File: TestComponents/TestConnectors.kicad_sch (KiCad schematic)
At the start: 9 parts, among them J2-1 Conn_01x04_Male, J2-2 Conn_01x04_Male

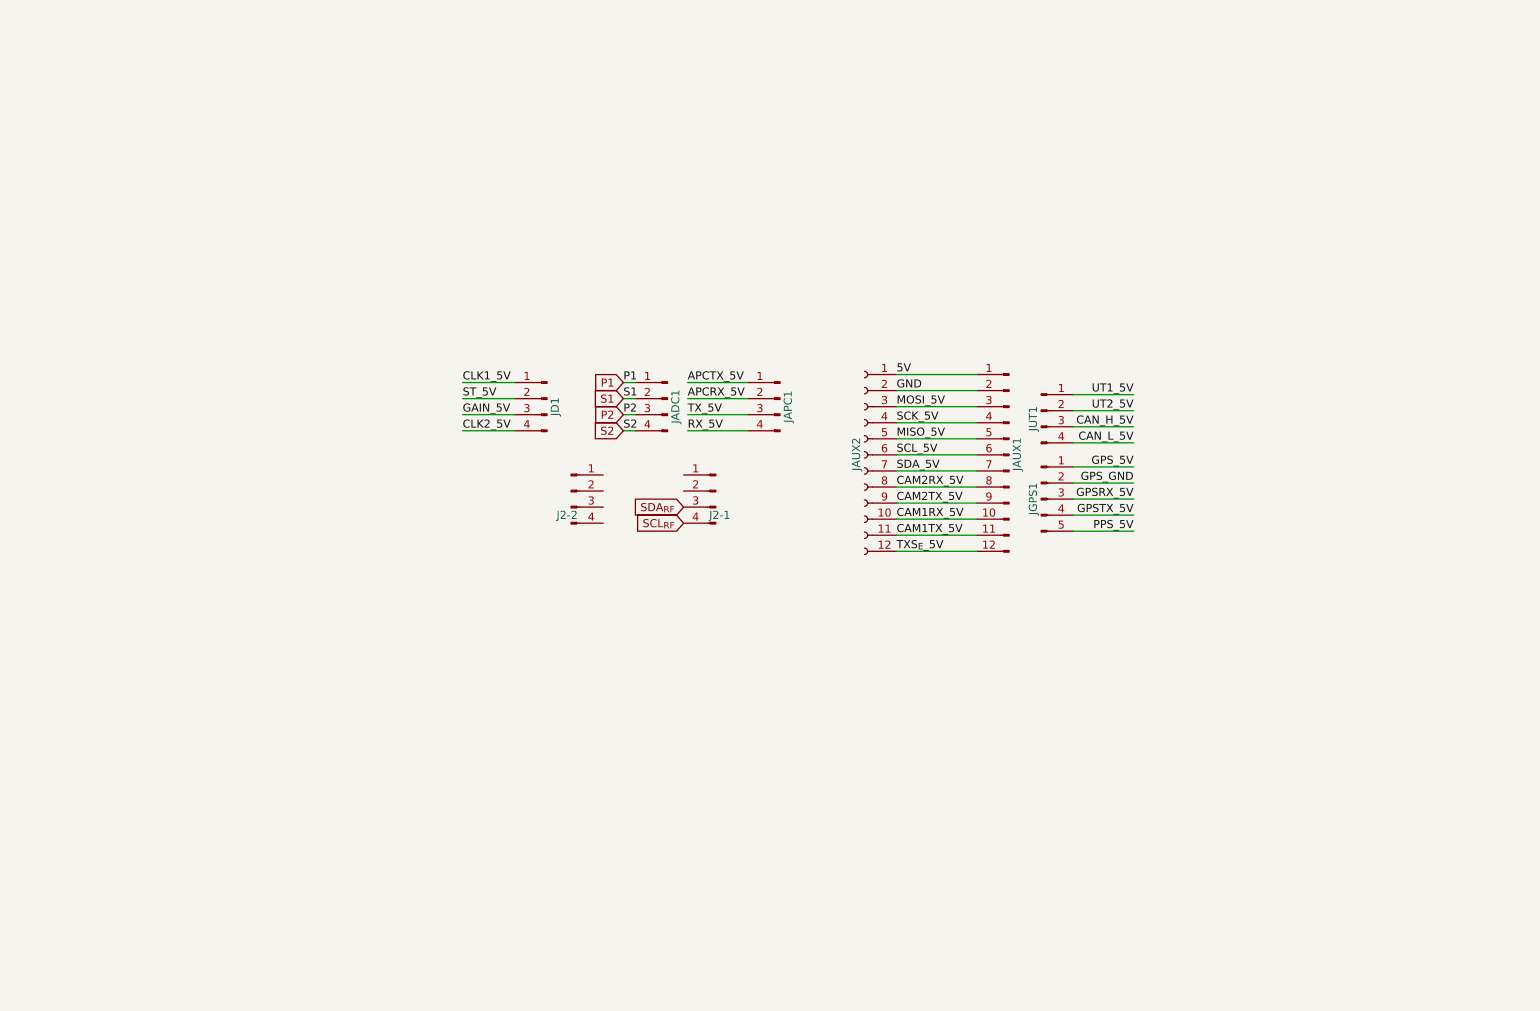
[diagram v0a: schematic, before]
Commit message: SpectDrone Development
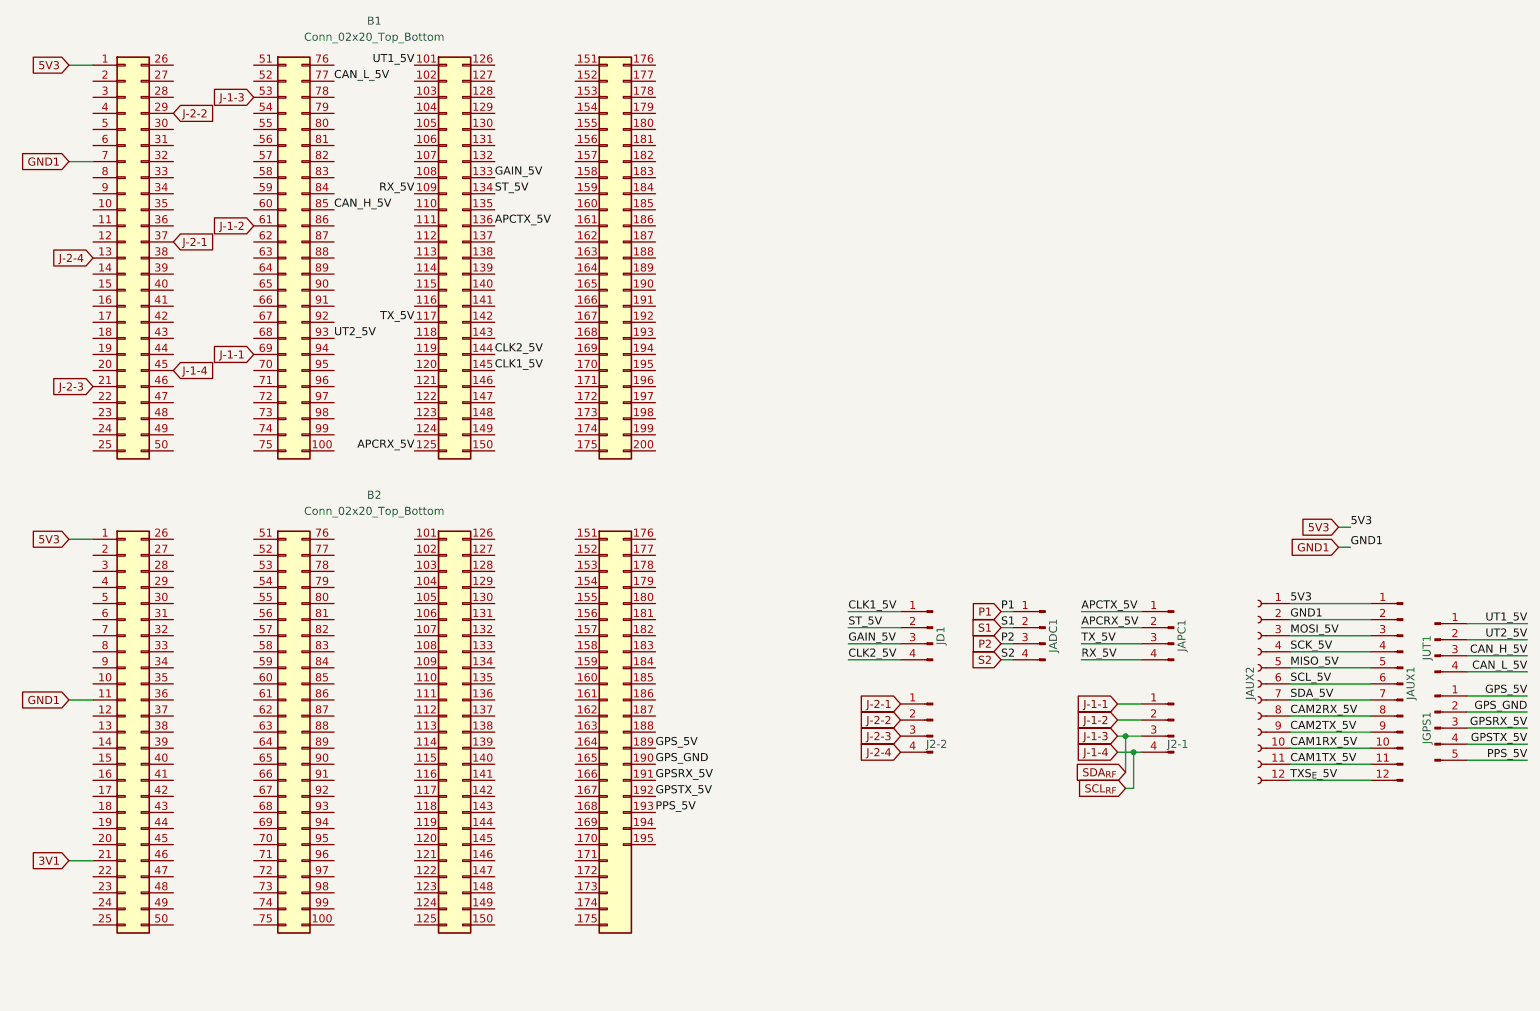
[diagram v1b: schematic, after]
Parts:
- added B1: Conn_02x20_Top_Bottom, Gardenuino Custom:PinHeader_CornerB1, symbol Connector_Generic:Conn_02x20_Top_Bottom
- added B2: Conn_02x20_Top_Bottom, Gardenuino Custom:PinHeader_CornerB2, symbol Connector_Generic:Conn_02x20_Top_Bottom
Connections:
- net APCRX_5V: now also B1.125 (Pin_125)
- net APCTX_5V: now also B1.136 (Pin_136)
- net CAN_H_5V: now also B1.85 (Pin_85)
- net CAN_L_5V: now also B1.77 (Pin_77)
- net CLK1_5V: now also B1.145 (Pin_145)
- net CLK2_5V: now also B1.144 (Pin_144)
- net GAIN_5V: now also B1.133 (Pin_133)
- net GPSRX_5V: now also B2.191 (Pin_191)
- net GPSTX_5V: now also B2.192 (Pin_192)
- net GPS_5V: now also B2.189 (Pin_189)
- net GPS_GND: now also B2.190 (Pin_190)
- net PPS_5V: now also B2.193 (Pin_193)
- net RX_5V: now also B1.109 (Pin_109)
- net ST_5V: now also B1.134 (Pin_134)
- net TX_5V: now also B1.117 (Pin_117)
- net UT1_5V: now also B1.101 (Pin_101)
- net UT2_5V: now also B1.93 (Pin_93)
- net J-2-1: now reaches J2-2.1 (Pin_1)
- net J-2-1: now also B1.37 (Pin_37)
- net J-2-2: now reaches J2-2.2 (Pin_2)
- net J-2-2: now also B1.29 (Pin_29)
- net J-2-3: now reaches J2-2.3 (Pin_3)
- net J-2-3: now also B1.21 (Pin_21)
- net J-2-4: now reaches J2-2.4 (Pin_4)
- net J-2-4: now also B1.13 (Pin_13)
- net J-1-1: now reaches J2-1.1 (Pin_1)
- net J-1-1: now also B1.69 (Pin_69)
- net J-1-2: now reaches J2-1.2 (Pin_2)
- net J-1-2: now also B1.61 (Pin_61)
- net 5V renamed 5V3
- net 5V3: now also B1.1 (Pin_1), B2.1 (Pin_1)
- net GND renamed GND1
- net GND1: now also B1.7 (Pin_7), B2.11 (Pin_11)
- net SCL_{RF} renamed J-1-4
- net J-1-4: now also B1.45 (Pin_45)
- net SDA_{RF} renamed J-1-3
- net J-1-3: now also B1.53 (Pin_53)
- new net 3V1: B2.21 (Pin_21)
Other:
- moved on the sheet: J2-1, J2-2, JADC1, JAPC1, JAUX1, JAUX2, JD1, JGPS1, JUT1

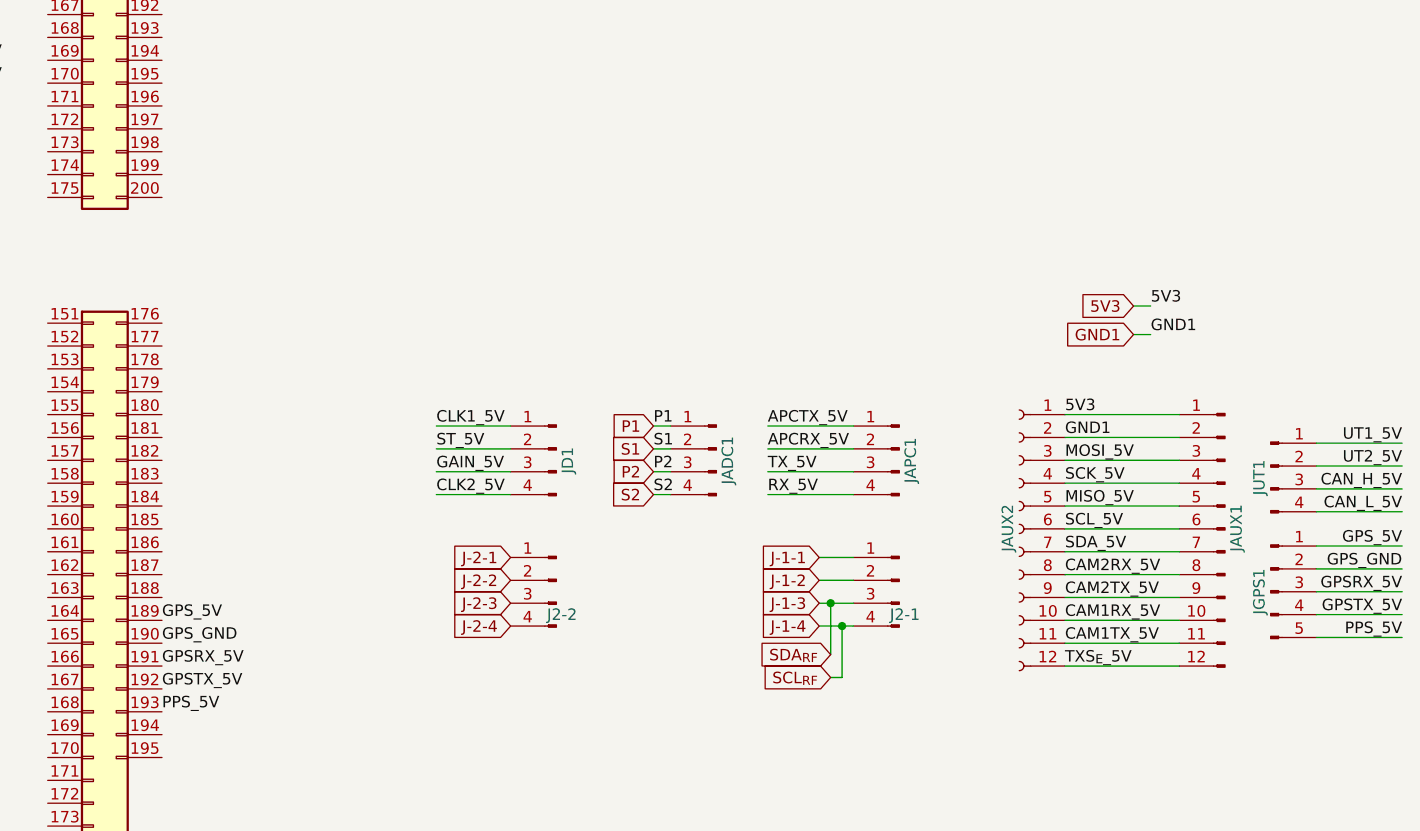
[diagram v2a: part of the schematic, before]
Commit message: SpectDrone Development
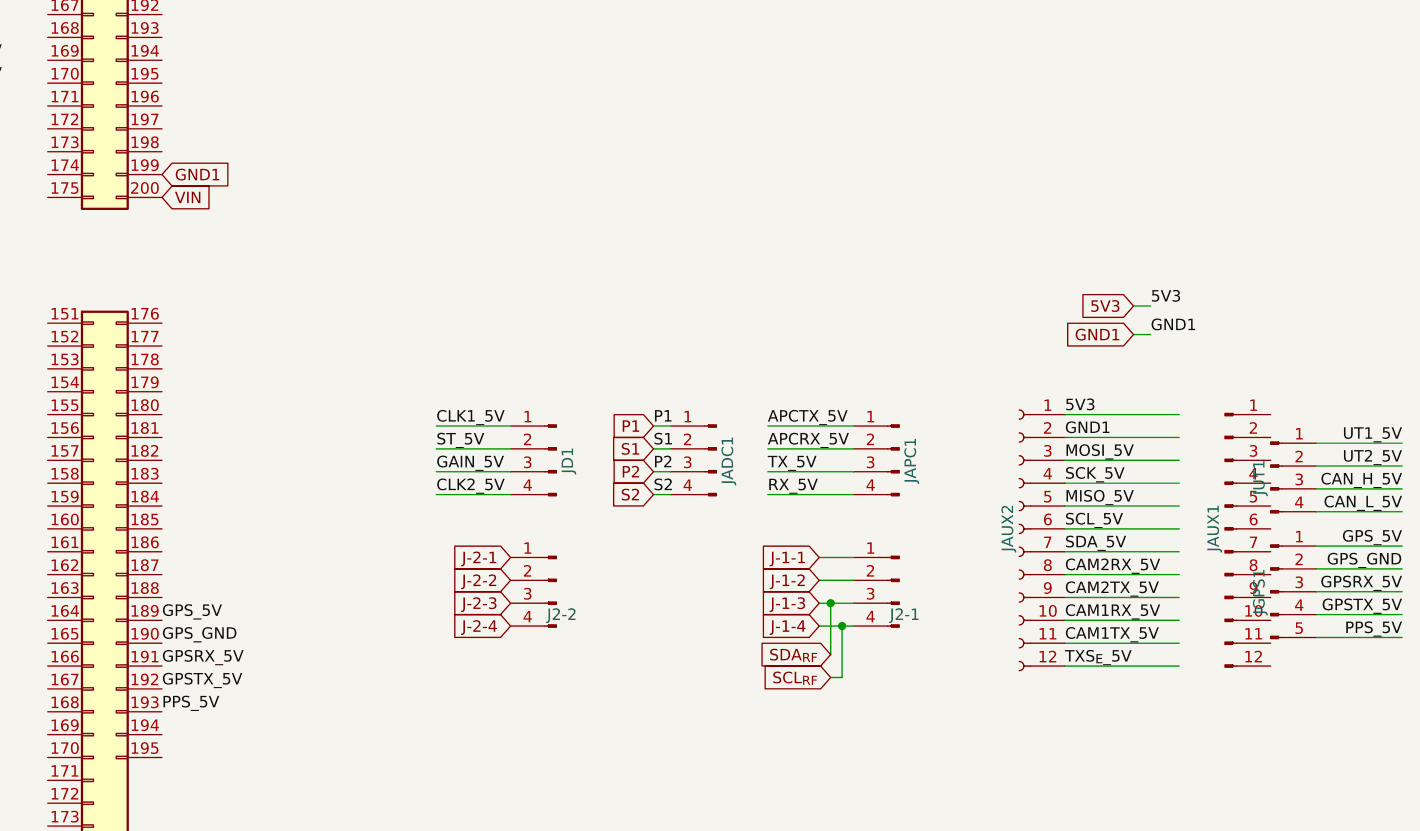
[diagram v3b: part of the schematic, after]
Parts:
- J2-1, J2-2, JADC1, JAPC1, JD1, JUT1: footprint Connector_PinSocket_2.54mm:PinSocket_1x04_P2.54mm_Vertical -> Connector_PinHeader_2.54mm:PinHeader_1x04_P2.54mm_Vertical
- JAUX1: footprint Connector_PinSocket_2.54mm:PinSocket_1x12_P2.54mm_Vertical -> Connector_PinHeader_2.54mm:PinHeader_1x12_P2.54mm_Vertical
- JGPS1: footprint Connector_PinSocket_2.54mm:PinSocket_1x05_P2.54mm_Vertical -> Connector_PinHeader_2.54mm:PinHeader_1x05_P2.54mm_Vertical
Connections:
- net 5V3: no longer JAUX1.1 (Pin_1)
- net CAM1RX_5V: no longer JAUX1.10 (Pin_10)
- net CAM1TX_5V: no longer JAUX1.11 (Pin_11)
- net CAM2RX_5V: no longer JAUX1.8 (Pin_8)
- net CAM2TX_5V: no longer JAUX1.9 (Pin_9)
- net GND1: now also B1.199 (Pin_199); no longer JAUX1.2 (Pin_2)
- net MISO_5V: no longer JAUX1.5 (Pin_5)
- net MOSI_5V: no longer JAUX1.3 (Pin_3)
- net SCK_5V: no longer JAUX1.4 (Pin_4)
- net SCL_5V: no longer JAUX1.6 (Pin_6)
- net SDA_5V: no longer JAUX1.7 (Pin_7)
- net TXS_{E}_5V: no longer JAUX1.12 (Pin_12)
- net VIN: now reaches B1.200 (Pin_200)
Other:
- moved on the sheet: JAUX1
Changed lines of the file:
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@@
+    )
+  )
+  (global_label "GND1" (shape input) (at 130.175 96.52 0) (fields_autoplaced)
+    (effects (font (size 1.27 1.27)) (justify left))
+    (property "Intersheet References" "${INTERSHEET_REFS}" (id 0) (at 137.6681 96.4406 0)
+      (effects (font (size 1.27 1.27)) (justify left) hide)
     )
   )
@@
     (property "Intersheet References" "${INTERSHEET_REFS}" (id 0) (at 196.6624 152.4794 0)
       (effects (font (size 1.27 1.27)) (justify right) hide)
+    )
+  )
+  (global_label "VIN" (shape input) (at 130.175 99.06 0) (fields_autoplaced)
+    (effects (font (size 1.27 1.27)) (justify left))
+    (property "Intersheet References" "${INTERSHEET_REFS}" (id 0) (at 135.6119 99.1394 0)
+      (effects (font (size 1.27 1.27)) (justify left) hide)
     )
   )
@@
       (effects (font (size 1.27 1.27)) hide)
     )
-    (property "Footprint" "Connector_PinSocket_2.54mm:PinSocket_1x04_P2.54mm_Vertical" (id 2) (at 173.99 127 0)
+    (property "Footprint" "Connector_PinHeader_2.54mm:PinHeader_1x04_P2.54mm_Vertical" (id 2) (at 173.99 127 0)
       (effects (font (size 1.27 1.27)) hide)
     )
@@
       (effects (font (size 1.27 1.27)) hide)
     )
-    (property "Footprint" "Connector_PinSocket_2.54mm:PinSocket_1x04_P2.54mm_Vertical" (id 2) (at 253.365 128.905 0)
+    (property "Footprint" "Connector_PinHeader_2.54mm:PinHeader_1x04_P2.54mm_Vertical" (id 2) (at 253.365 128.905 0)
       (effects (font (size 1.27 1.27)) hide)
     )
@@
       (effects (font (size 1.27 1.27)) hide)
     )
-    (property "Footprint" "Connector_PinSocket_2.54mm:PinSocket_1x04_P2.54mm_Vertical" (id 2) (at 173.99 141.605 0)
+    (property "Footprint" "Connector_PinHeader_2.54mm:PinHeader_1x04_P2.54mm_Vertical" (id 2) (at 173.99 141.605 0)
       (effects (font (size 1.27 1.27)) hide)
     )
@@
       (effects (font (size 1.27 1.27)) (justify left) hide)
     )
-    (property "Footprint" "Connector_PinSocket_2.54mm:PinSocket_1x05_P2.54mm_Vertical" (id 2) (at 253.365 142.875 0)
+    (property "Footprint" "Connector_PinHeader_2.54mm:PinHeader_1x05_P2.54mm_Vertical" (id 2) (at 253.365 142.875 0)
       (effects (font (size 1.27 1.27)) hide)
     )
@@
       (effects (font (size 1.27 1.27)) hide)
     )
-    (property "Footprint" "Connector_PinSocket_2.54mm:PinSocket_1x04_P2.54mm_Vertical" (id 2) (at 212.09 127 0)
+    (property "Footprint" "Connector_PinHeader_2.54mm:PinHeader_1x04_P2.54mm_Vertical" (id 2) (at 212.09 127 0)
       (effects (font (size 1.27 1.27)) hide)
     )
@@
       (effects (font (size 1.27 1.27)) hide)
     )
-    (property "Footprint" "Connector_PinSocket_2.54mm:PinSocket_1x04_P2.54mm_Vertical" (id 2) (at 191.77 127 0)
+    (property "Footprint" "Connector_PinHeader_2.54mm:PinHeader_1x04_P2.54mm_Vertical" (id 2) (at 191.77 127 0)
       (effects (font (size 1.27 1.27)) hide)
     )
@@
       (effects (font (size 1.27 1.27)) hide)
     )
-    (property "Footprint" "Connector_PinSocket_2.54mm:PinSocket_1x04_P2.54mm_Vertical" (id 2) (at 212.09 141.605 0)
+    (property "Footprint" "Connector_PinHeader_2.54mm:PinHeader_1x04_P2.54mm_Vertical" (id 2) (at 212.09 141.605 0)
       (effects (font (size 1.27 1.27)) hide)
     )
@@
     (pin "4")
   )
-  (symbol (lib_id "Connector:Conn_01x12_Male") (at 248.285 135.89 0) (mirror y) (unit 1)
-    (in_bom yes) (on_board yes)
-    (property "Reference" "JAUX1" (id 0) (at 249.555 138.43 90)
+  (symbol (lib_id "Connector:Conn_01x12_Male") (at 248.285 135.89 0) (unit 1)
+    (in_bom yes) (on_board yes)
+    (property "Reference" "JAUX1" (id 0) (at 247.015 138.43 90)
       (effects (font (size 1.27 1.27)) (justify left))
     )
-    (property "Value" "AUX" (id 1) (at 250.825 137.16 90)
+    (property "Value" "AUX" (id 1) (at 245.745 137.16 90)
       (effects (font (size 1.27 1.27)) (justify left) hide)
     )
-    (property "Footprint" "Connector_PinSocket_2.54mm:PinSocket_1x12_P2.54mm_Vertical" (id 2) (at 248.285 135.89 0)
-      (effects (font (size 1.27 1.27)) hide)
-    )
+    (property "Footprint" "Connector_PinHeader_2.54mm:PinHeader_1x12_P2.54mm_Vertical" (id 2) (at 248.285 135.89 0)
+      (effects (font (size 1.27 1.27)) hide)
+    )
